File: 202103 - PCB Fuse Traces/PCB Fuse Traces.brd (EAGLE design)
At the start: 8 parts

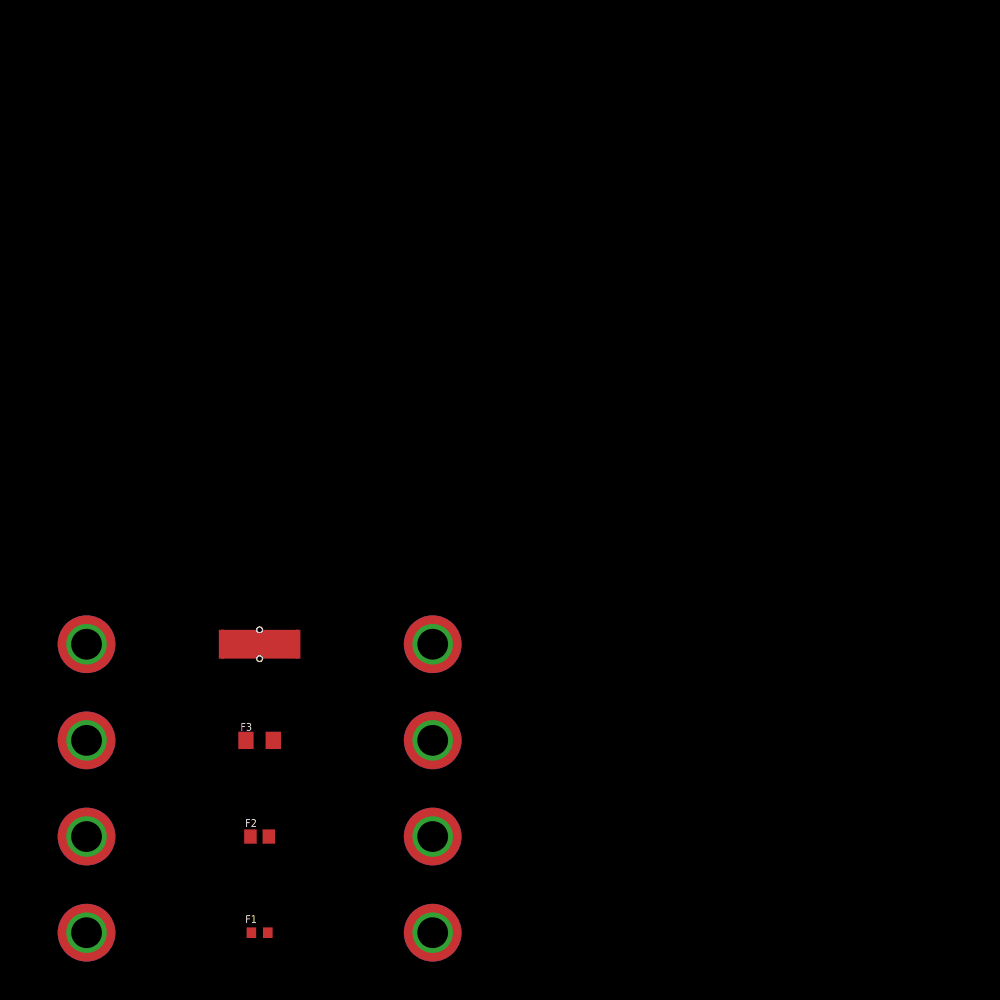
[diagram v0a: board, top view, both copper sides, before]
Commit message: 20210315
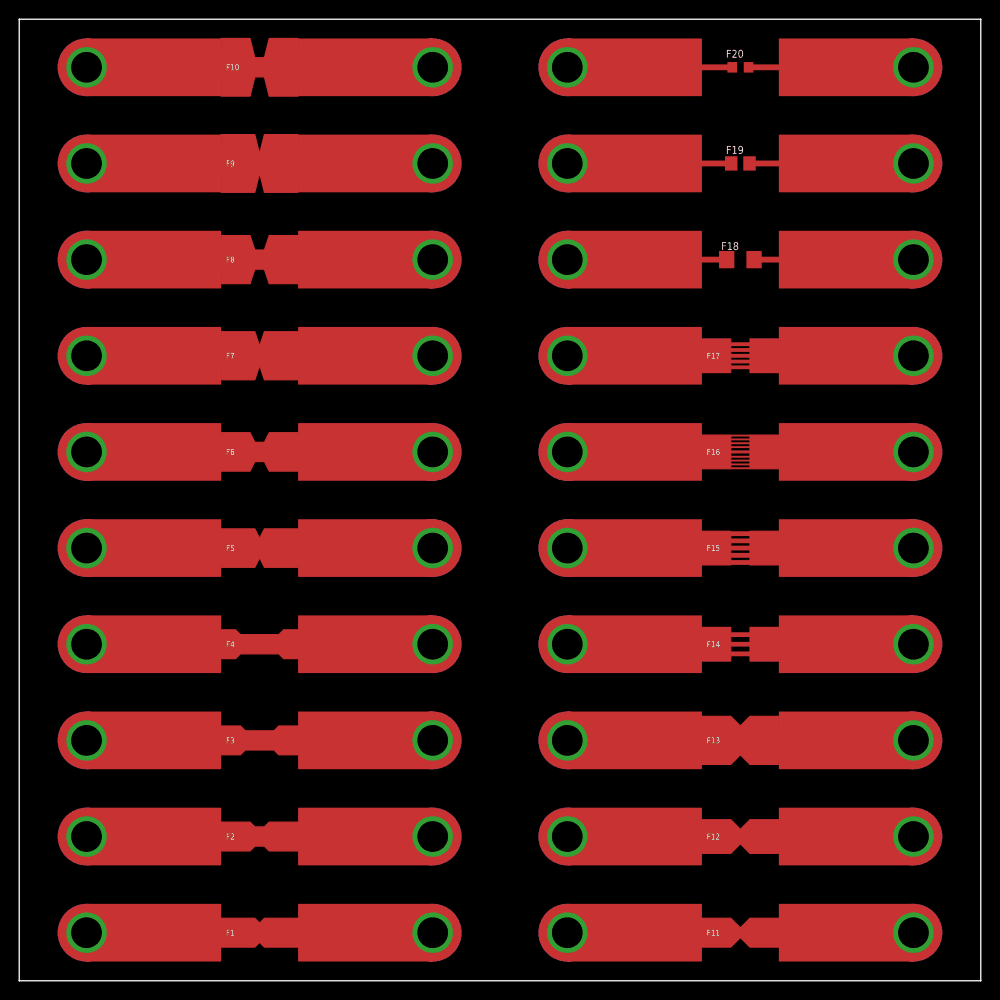
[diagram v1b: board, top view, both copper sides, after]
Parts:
- added F10: (no value), nolan:FUSE_DD
- added F11: (no value), nolan:FUSE_A0
- added F12: (no value), nolan:FUSE_A1
- added F13: (no value), nolan:FUSE_A3
- added F14: (no value), nolan:FUSE_B1
- added F15: (no value), nolan:FUSE_B2
- added F16: (no value), nolan:FUSE_B3
- added F17: (no value), nolan:FUSE_B4
- added F18: (no value), nolan:F1206
- added F19: (no value), nolan:F0805
- added F20: (no value), nolan:F0603
- added F5: (no value), nolan:FUSE_B
- added F6: (no value), nolan:FUSE_BB
- added F7: (no value), nolan:FUSE_C
- added F8: (no value), nolan:FUSE_CC
- added F9: (no value), nolan:FUSE_D
- added FH10, FH11, FH12, FH13, FH14, FH15, FH16, FH17, FH18, FH19, FH20, FH5, FH6, FH7, FH8, FH9: (no value), nolan:F36_HOLDER
- F1: device nolan:F0603 -> nolan:FUSE_A
- F2: device nolan:F0805 -> nolan:FUSE_AA
- F3: device nolan:F1206 -> nolan:FUSE_AAA
- F4: device nolan:FUSE_100A -> nolan:FUSE_AAAA
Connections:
- new net N$10: F6.1, FH6.1
- new net N$11: F7.1, FH7.1
- new net N$12: F8.1, FH8.1
- new net N$13: F5.2, FH5.2
- new net N$14: F6.2, FH6.2
- new net N$15: F7.2, FH7.2
- new net N$16: F8.2, FH8.2
- new net N$17: F9.1, FH9.1
- new net N$18: F10.1, FH10.1
- new net N$19: F11.3, FH11.1
- new net N$20: F12.1, FH12.1
- new net N$21: F9.2, FH9.2
- new net N$22: F10.2, FH10.2
- new net N$23: F11.4, FH11.2
- new net N$24: F12.2, FH12.2
- new net N$25: F13.1, FH13.1
- new net N$26: F14.1, FH14.1
- new net N$27: F15.1, FH15.1
- new net N$28: F16.1, FH16.1
- new net N$29: F13.2, FH13.2
- new net N$30: F14.2, FH14.2
- new net N$31: F15.2, FH15.2
- new net N$32: F16.2, FH16.2
- new net N$33: F17.1, FH17.1
- new net N$34: F18.1, FH18.1
- new net N$35: F19.1, FH19.1
- new net N$36: F20.1, FH20.1
- new net N$37: F17.2, FH17.2
- new net N$38: F18.2, FH18.2
- new net N$39: F19.2, FH19.2
- new net N$40: F20.2, FH20.2
- new net N$9: F5.1, FH5.1
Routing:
- net N$40: track 0.00 -> 17.2 mm
- net N$36: track 0.00 -> 17.2 mm
- net N$39: track 0.00 -> 17.0 mm
- net N$35: track 0.00 -> 17.0 mm
- net N$38: track 0.00 -> 16.6 mm
- net N$34: track 0.00 -> 16.6 mm
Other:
- board outline added: 100 x 100 mm
